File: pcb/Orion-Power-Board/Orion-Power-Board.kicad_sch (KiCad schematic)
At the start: 20 parts, among them J1 2S_FRONT_BATTERY_BALANCE_HEAD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, J2 2S_BACK_BATTERY_BALANCE_HEADER, J3 3S_BATTERY_BALANCE_HEADER, J4 CONN_20_POS_KEYED_SOCKET, J5 2S_FRONT_LI-ION_VOLTAGE_ALARM, J6 2S_BACK_LI-ION_VOLTAGE_ALARM, J7 3S_LI-ION_VOLTAGE_ALARM, U1 FRONT_6x3_SERVO_HEADER_PIN, U2 BACK_6x3_SERVO_HEADER_PIN

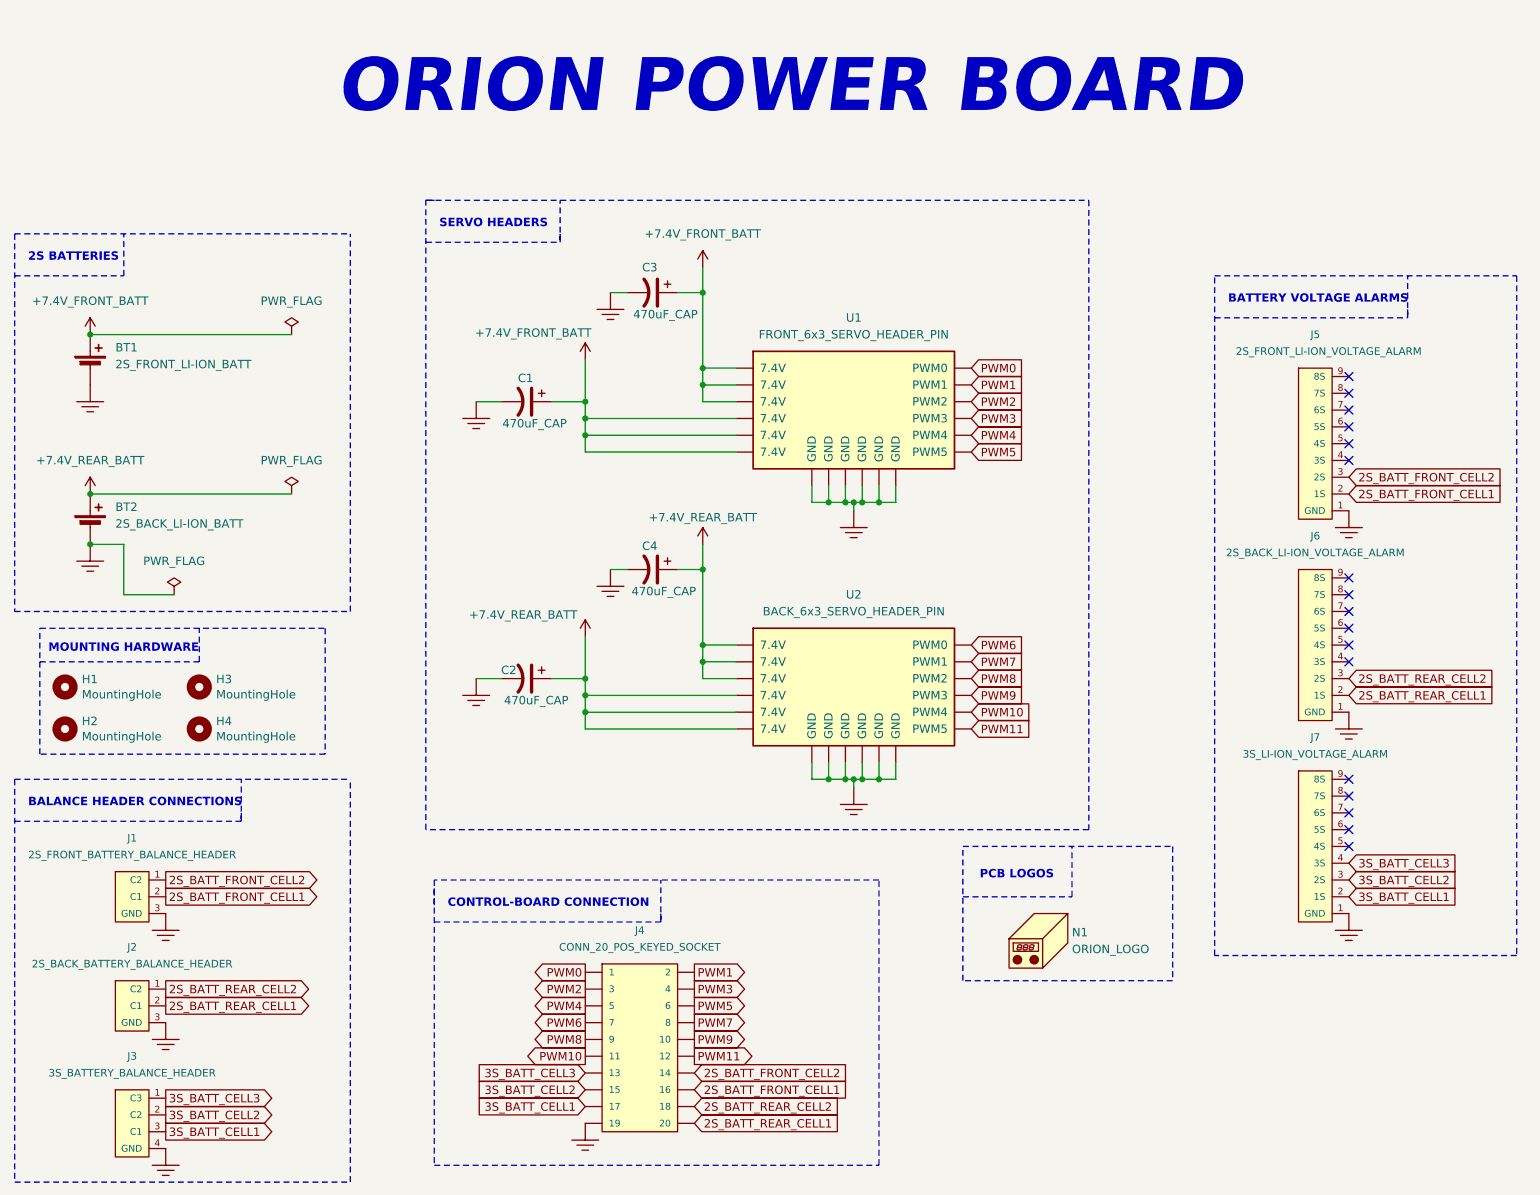
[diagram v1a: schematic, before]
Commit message: Update schematics
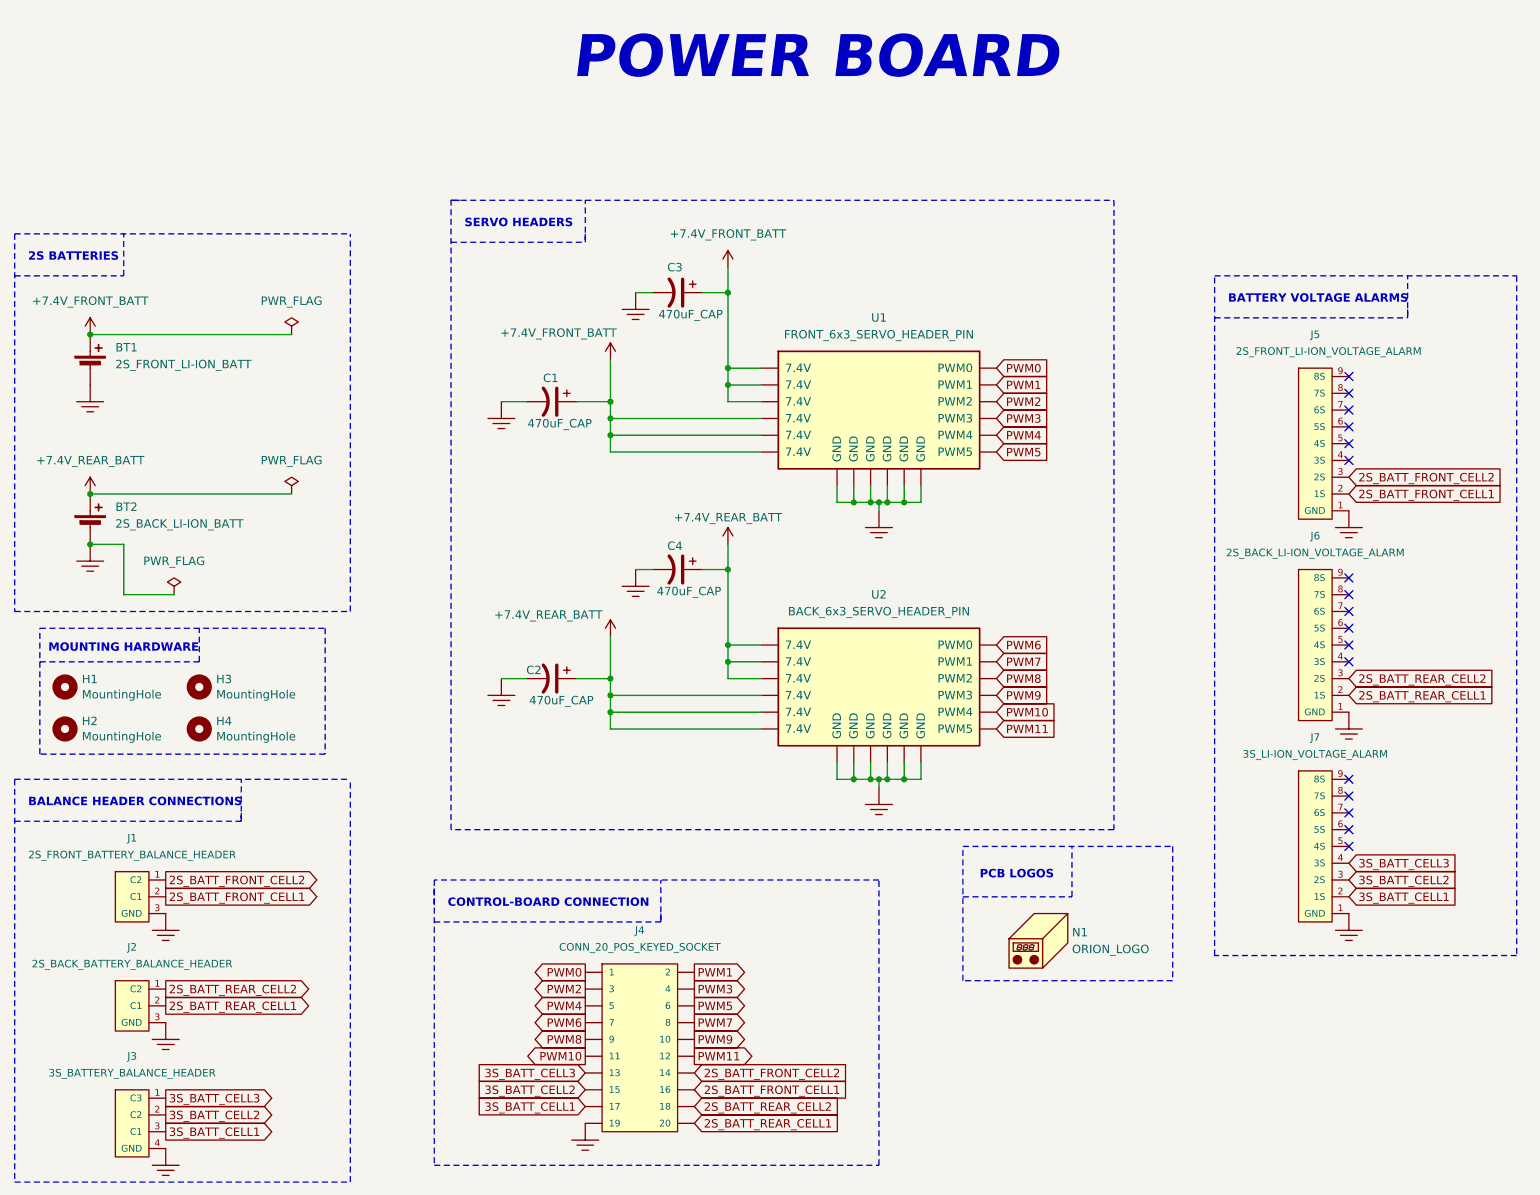
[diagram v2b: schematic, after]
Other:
- note added: "POWER BOARD"
- note removed: "ORION POWER BOARD"
- moved on the sheet: C1, C2, C3, C4, U1, U2
